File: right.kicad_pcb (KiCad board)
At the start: 2 copper layers, 152.4 x 109.7 mm, 51 parts, among them J1 Conn_01x07, J2 Conn_01x07, U1 74VHC4051AFT, U2 GS8051-TR

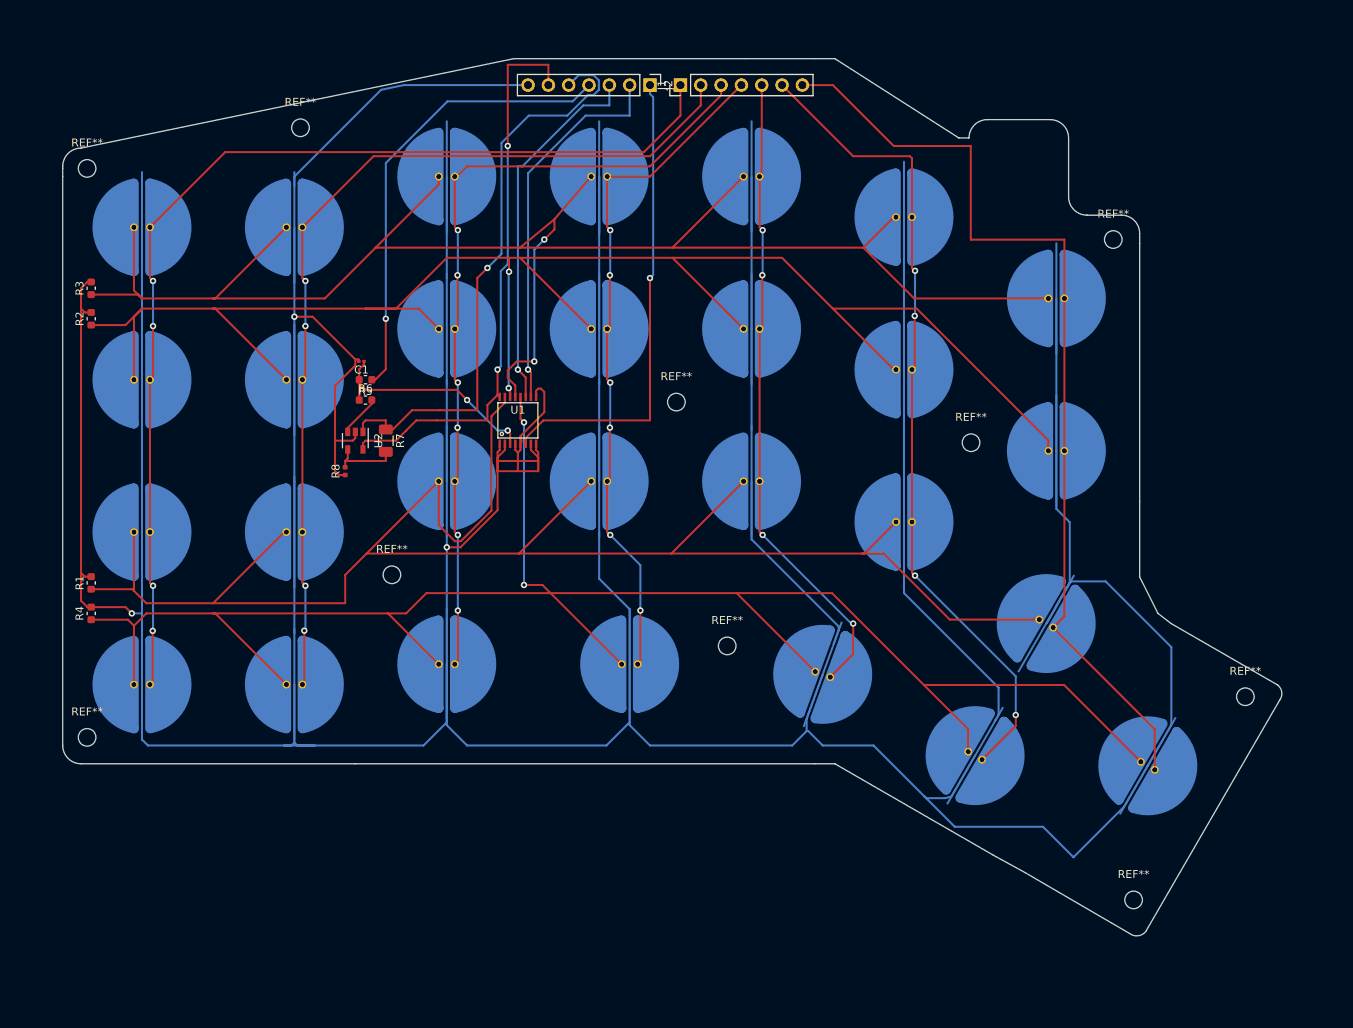
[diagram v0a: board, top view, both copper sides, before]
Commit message: add zone
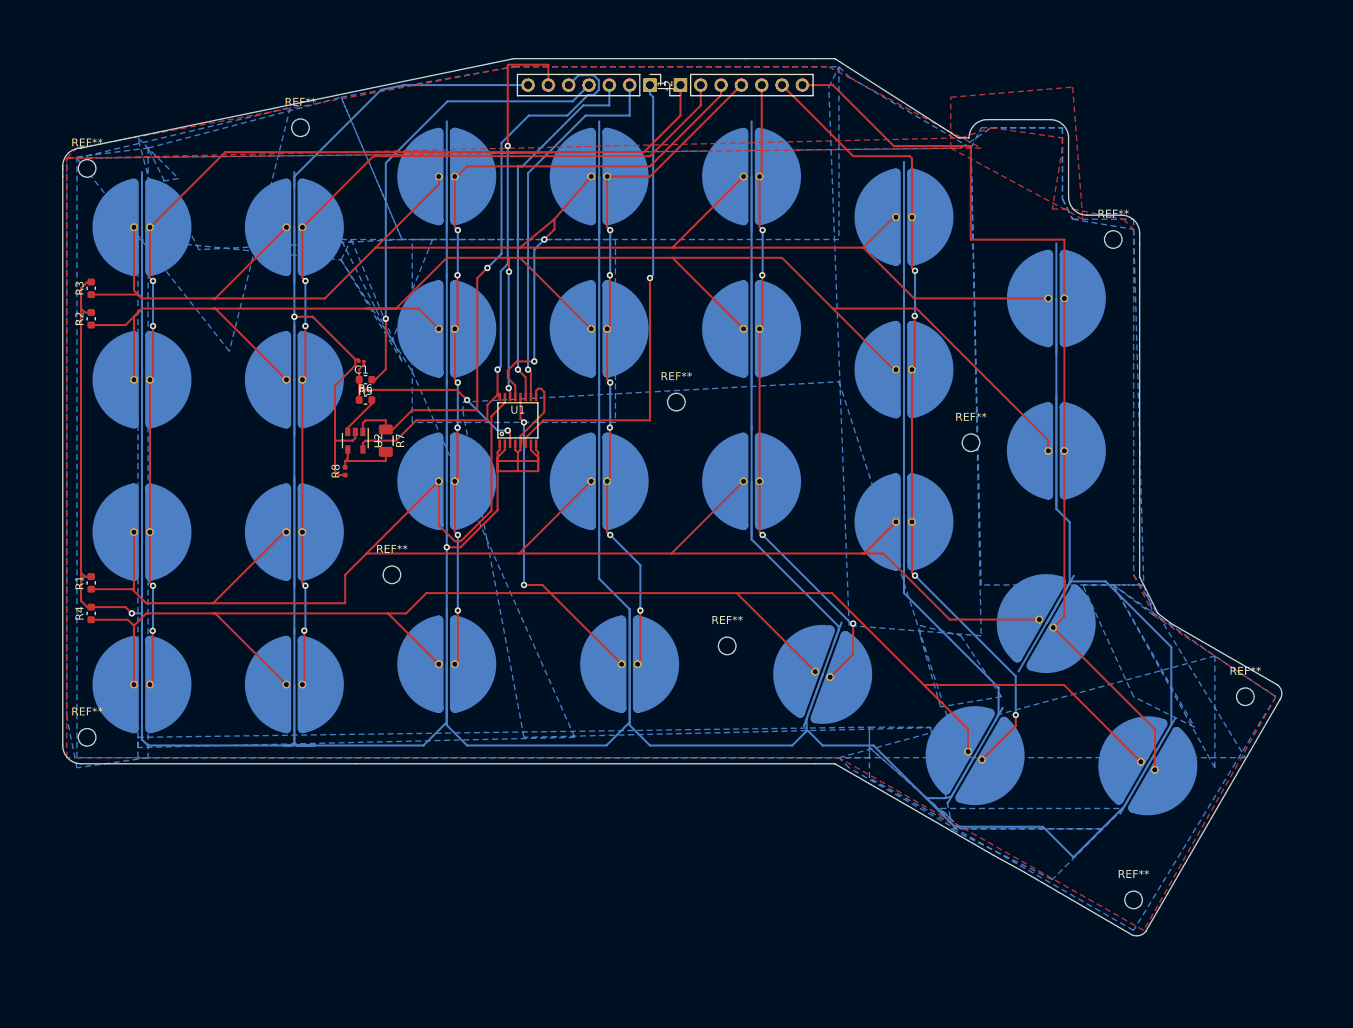
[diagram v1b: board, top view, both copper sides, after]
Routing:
- added copper zone on B.Cu, net GND
- added copper zone on F.Cu, net GND

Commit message: clean up & add script
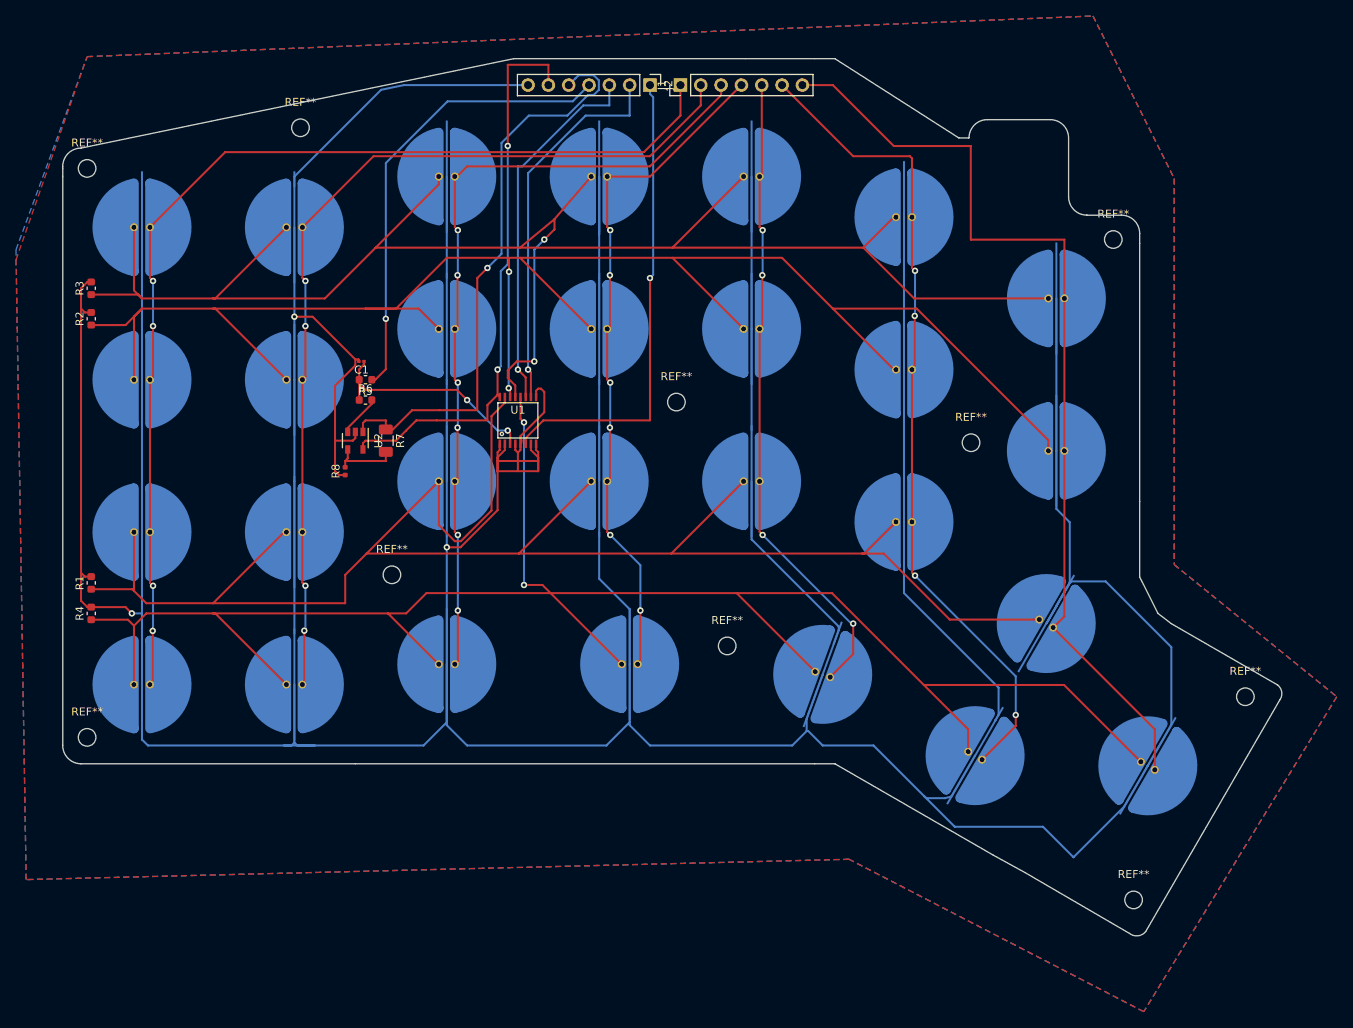
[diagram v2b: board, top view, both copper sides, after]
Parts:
- TP1, TP10, TP11, TP12, TP13, TP14, TP15, TP16, TP17, TP18, TP19, TP2, TP20, TP21, TP22, TP23, TP24, TP25, TP26, TP27, TP28, TP3, TP4, TP5, TP6, TP7, TP8, TP9: footprint lib:ToprePad -> base:ToprePad
- U1: footprint gsg-modules:TSSOP16 -> base:TSSOP16
